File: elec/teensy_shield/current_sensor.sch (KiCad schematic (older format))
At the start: 0 parts

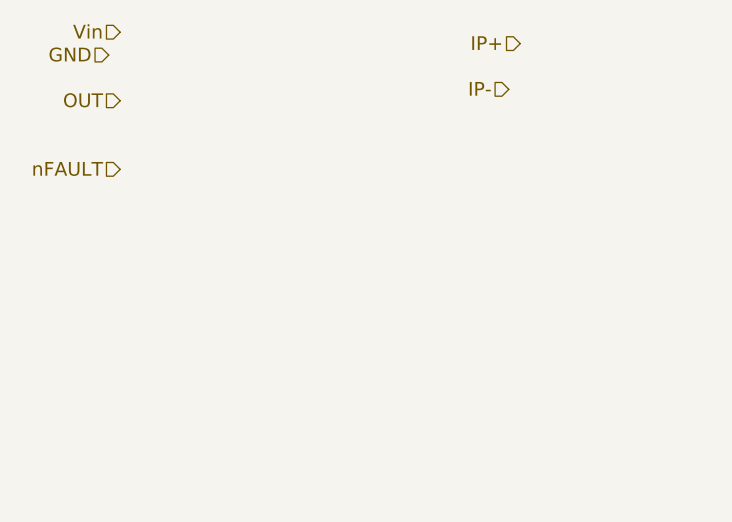
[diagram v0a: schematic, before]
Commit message: Completed new board schematics.
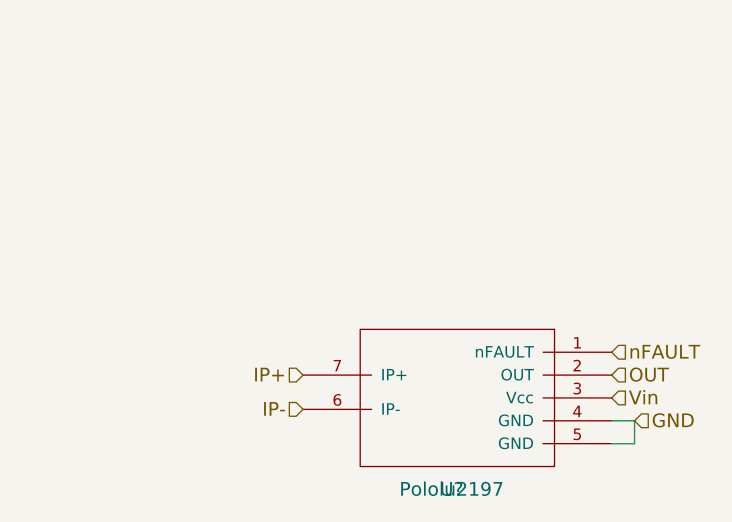
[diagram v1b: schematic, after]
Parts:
- added U?: Pololu2197, symbol Pololu2197
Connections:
- net GND: now also U?.4 (GND), U?.5 (GND)
- net IP+: now also U?.7 (IP+)
- net IP-: now also U?.6 (IP-)
- net OUT: now also U?.2 (OUT)
- net Vin: now also U?.3 (Vcc)
- net nFAULT: now also U?.1 (nFAULT)
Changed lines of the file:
@@
 LIBS:contrib
 LIBS:valves
+LIBS:arduino_shieldsNCL
+LIBS:teensy
+LIBS:pololu
+LIBS:teensy_shield-cache
 EELAYER 24 0
 EELAYER END
 $Descr A4 11693 8268
 encoding utf-8
-Sheet 6 26
+Sheet 6 34
 Title ""
 Date ""
@@
 Comment4 ""
 $EndDescr
-Text HLabel 4350 2250 0    60   Input ~ 0
+Text HLabel 6500 3850 2    60   Input ~ 0
 Vin
-Text HLabel 4300 2350 0    60   Input ~ 0
+Text HLabel 6600 3950 2    60   Input ~ 0
 GND
-Text HLabel 4350 2550 0    60   Input ~ 0
+Text HLabel 6500 3750 2    60   Input ~ 0
 OUT
-Text HLabel 4350 2850 0    60   Input ~ 0
+Text HLabel 6500 3650 2    60   Input ~ 0
 nFAULT
-Text HLabel 6100 2300 0    60   Input ~ 0
+Text HLabel 5150 3750 0    60   Input ~ 0
 IP+
-Text HLabel 6050 2500 0    60   Input ~ 0
+Text HLabel 5150 3900 0    60   Input ~ 0
 IP-
+$Comp
+L Pololu2197 U?
+U 1 1 55E8283A
+P 5800 3800
+F 0 "U?" H 5800 3350 60  0000 C CNN
+F 1 "Pololu2197" H 5800 3350 60  0000 C CNN
+F 2 "" H 5800 3350 60  0000 C CNN
+F 3 "" H 5800 3350 60  0000 C CNN
+	1    5800 3800
+	1    0    0    -1
+$EndComp
+Wire Wire Line
+	6500 3950 6600 3950
+Wire Wire Line
+	6600 3950 6600 4050
+Wire Wire Line
+	6600 4050 6500 4050
 $EndSCHEMATC

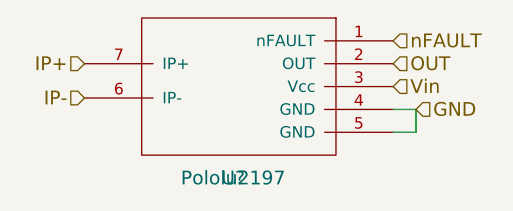
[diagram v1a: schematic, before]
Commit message: Elec ?
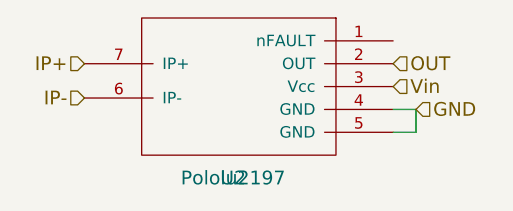
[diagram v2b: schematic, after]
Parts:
- gave numbers to parts that had none: 1
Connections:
- net nFAULT: no longer names the net of U11.1 (nFAULT)
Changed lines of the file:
@@
 Text HLabel 6500 3750 2    60   Input ~ 0
 OUT
-Text HLabel 6500 3650 2    60   Input ~ 0
-nFAULT
 Text HLabel 5150 3750 0    60   Input ~ 0
 IP+
@@
 IP-
 $Comp
-L Pololu2197 U?
+L Pololu2197 U11
 U 1 1 55E8283A
 P 5800 3800
-F 0 "U?" H 5800 3350 60  0000 C CNN
+AR Path="/55E6307C/55E63158/55E8283A" Ref="U11"  Part="1"
+AR Path="/55E7381B/55E63158/55E8283A" Ref="U2"  Part="1"
+AR Path="/55E7381C/55E63158/55E8283A" Ref="U5"  Part="1"
+AR Path="/55E7381D/55E63158/55E8283A" Ref="U8"  Part="1"
+F 0 "U2" H 5800 3350 60  0000 C CNN
 F 1 "Pololu2197" H 5800 3350 60  0000 C CNN
 F 2 "" H 5800 3350 60  0000 C CNN
